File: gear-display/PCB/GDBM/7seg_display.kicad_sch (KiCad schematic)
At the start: 13 parts

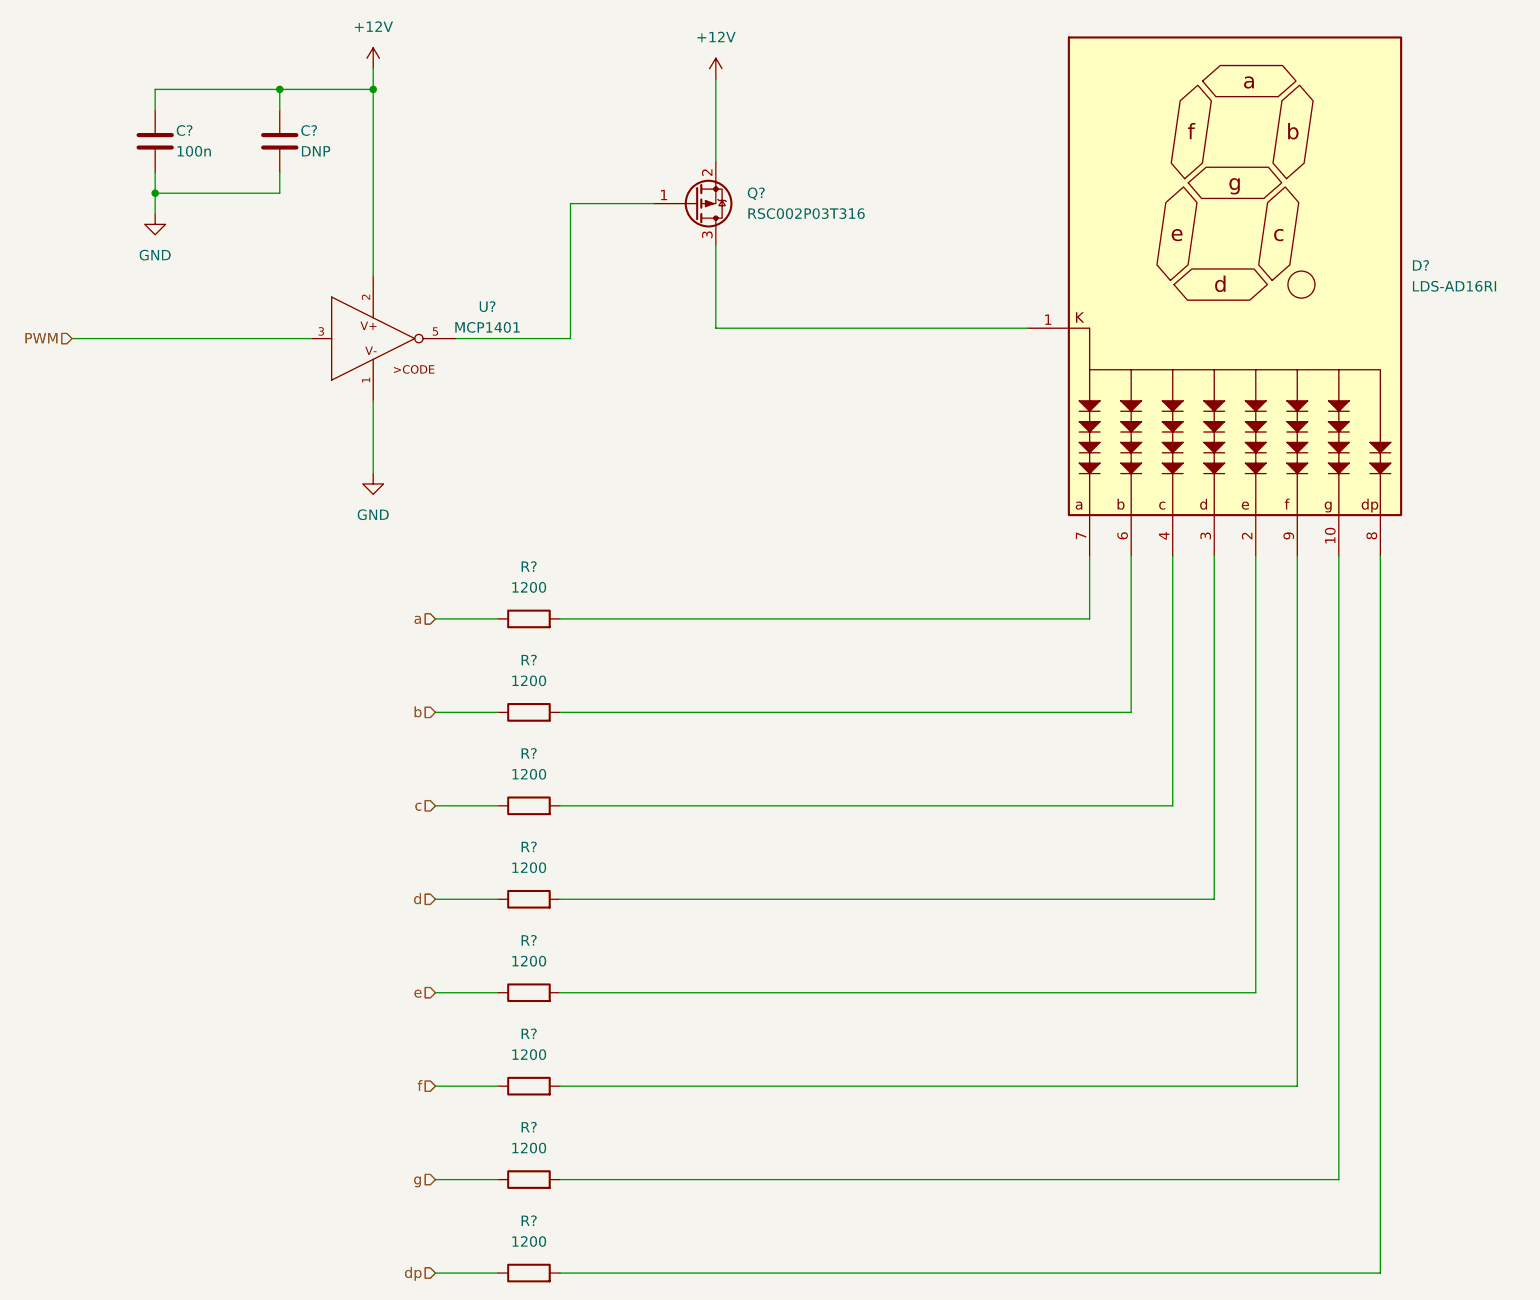
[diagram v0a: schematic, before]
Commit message: new features
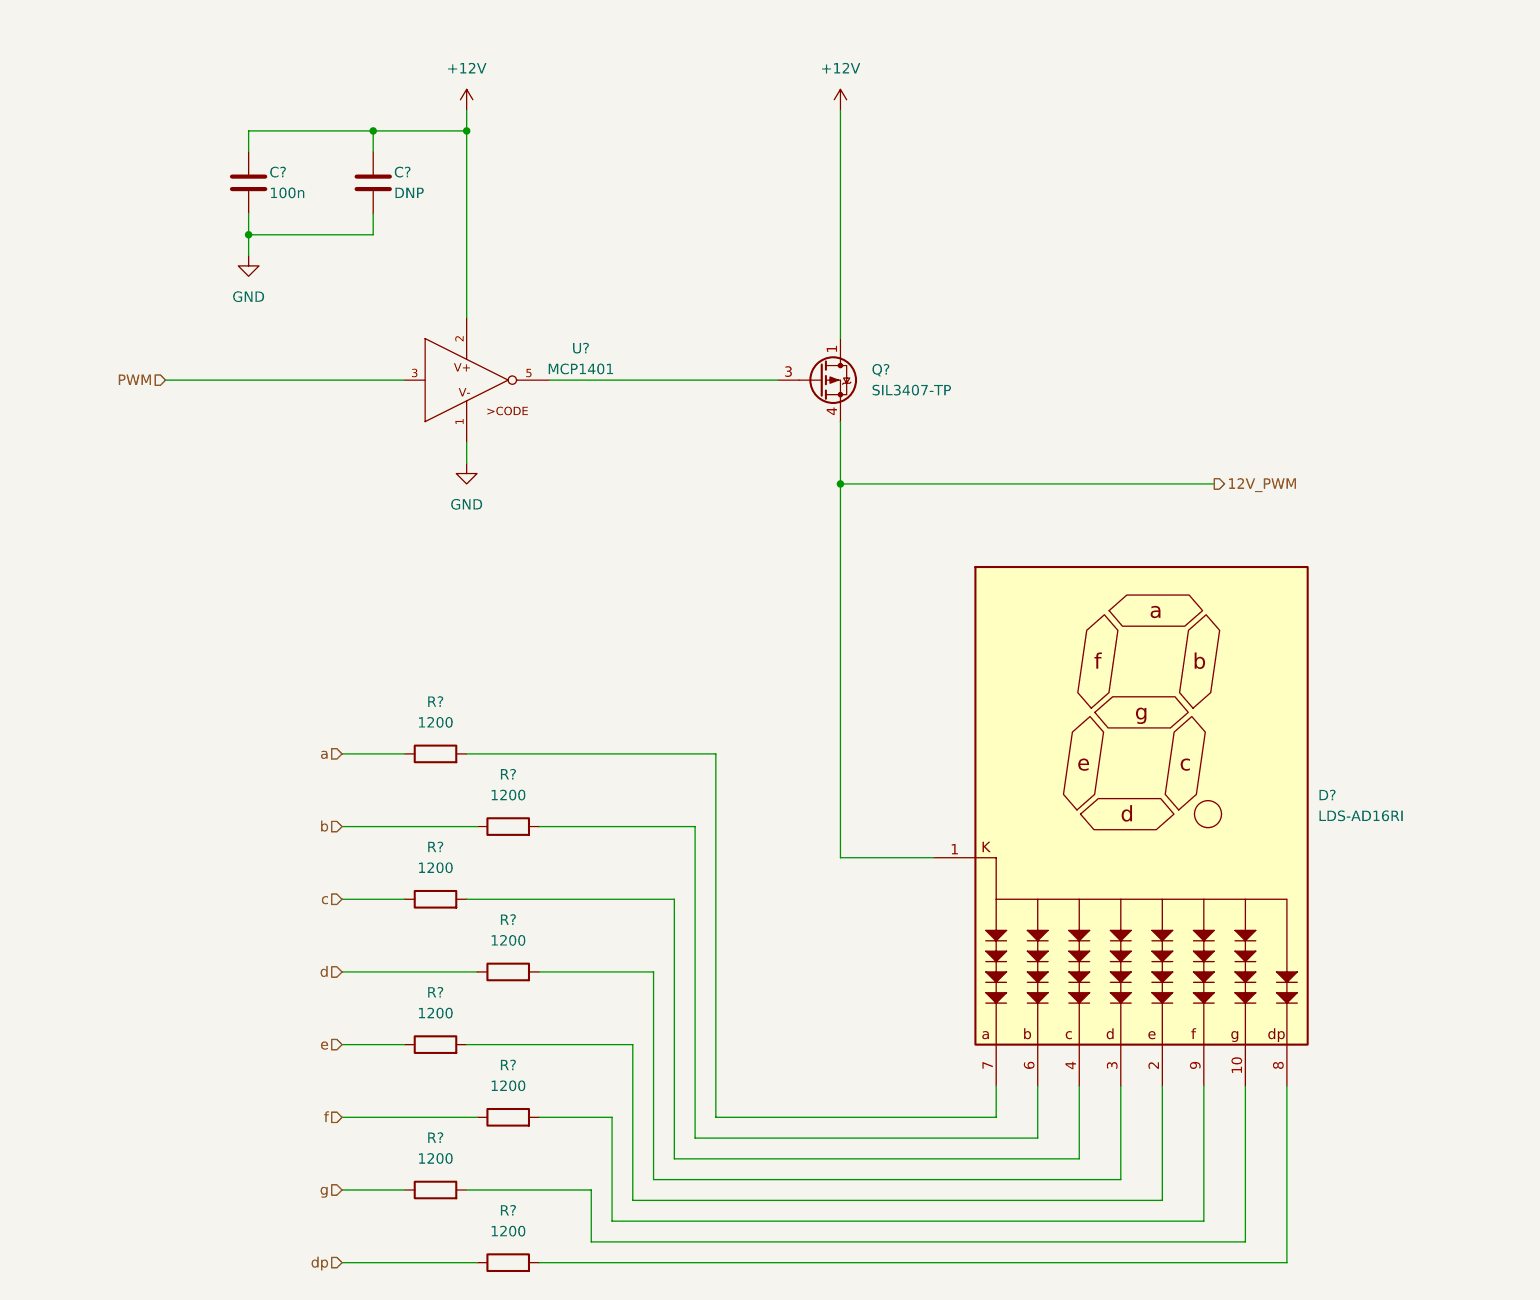
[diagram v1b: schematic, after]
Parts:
- removed Q?: PMOS_30V_250mA_RSC002P03T316, KD_Package_TO_SOT_SMD:SOT95P230X100-3N, symbol KD_Transistor_FET:PMOS_30V_250mA_RSC002P03T316
- added Q?: PMOS_30V_4A1_SIL3407-TP, KD_Package_TO_SOT_SMD:SOT95P280X120-6RN, symbol KD_Transistor_FET:PMOS_30V_4A1_SIL3407-TP
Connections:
- net +12V: now also Q?.1 (D), Q?.2 (D), Q?.5 (D), Q?.6 (D)
- net 12V_PWM: now reaches D?.1 (K), D?.5 (C)
- net 12V_PWM: now also Q?.4 (S)
- net at U?.5 (OUT): now also Q?.3 (G)
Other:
- moved on the sheet: C?, D?, R?, U?

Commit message: updates
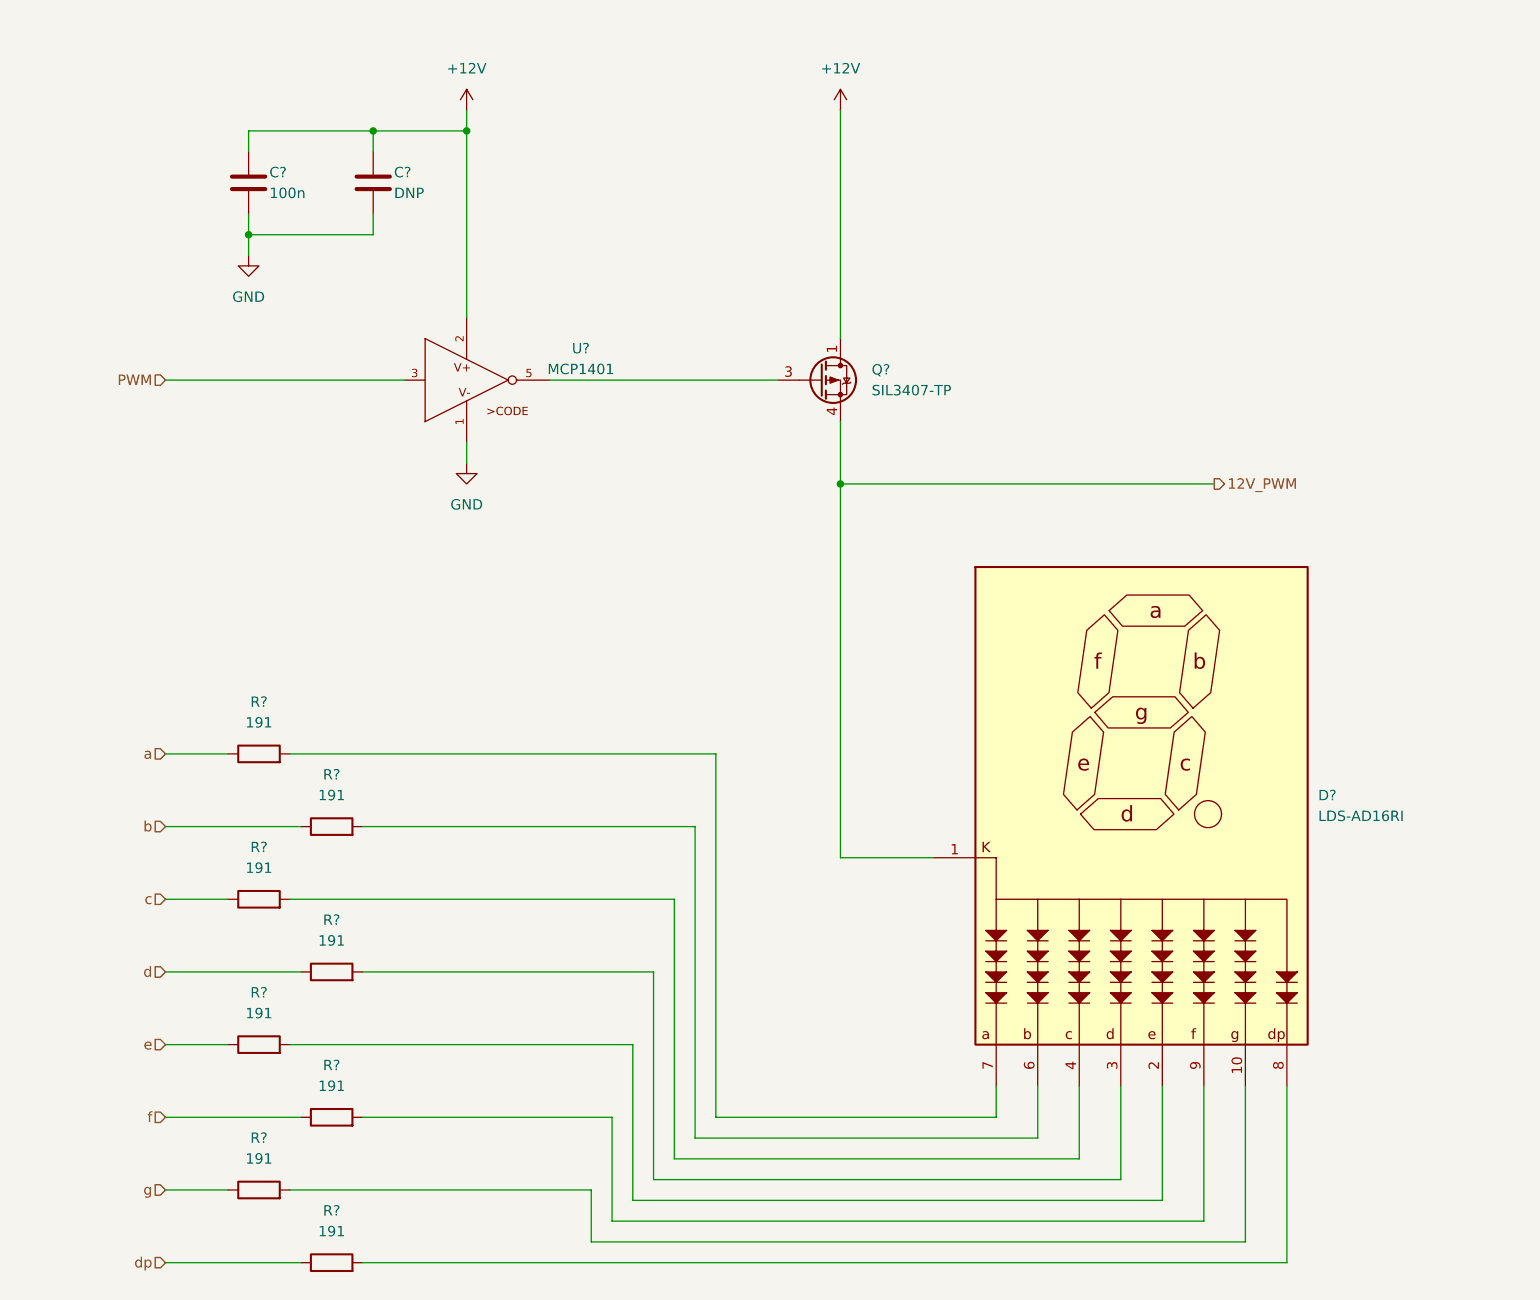
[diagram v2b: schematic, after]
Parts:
- removed R? (x8): R_0805_1200_5%, KD_Resistor:R_0805_2012Metric, symbol KD_Resistor:R_0805_1200_5%
- added R? (x8): R_1206_191_1%, KD_Resistor:RESC3216X70N, symbol KD_Resistor:R_1206_191_1%
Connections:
- net a: now also R?.1
- net b: now also R?.1
- net c: now also R?.1
- net d: now also R?.1
- net dp: now also R?.1
- net e: now also R?.1
- net f: now also R?.1
- net g: now also R?.1
- net at D?.7 (Aa): now also R?.2
- net at D?.2 (Ae): now also R?.2
- net at D?.10 (Ag): now also R?.2
- net at D?.3 (Ad): now also R?.2
- net at D?.4 (Ac): now also R?.2
- net at D?.6 (Ab): now also R?.2
- net at D?.8 (Adp): now also R?.2
- net at D?.9 (Af): now also R?.2
